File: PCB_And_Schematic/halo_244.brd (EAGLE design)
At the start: 38.1 x 42.9 mm, 14 parts

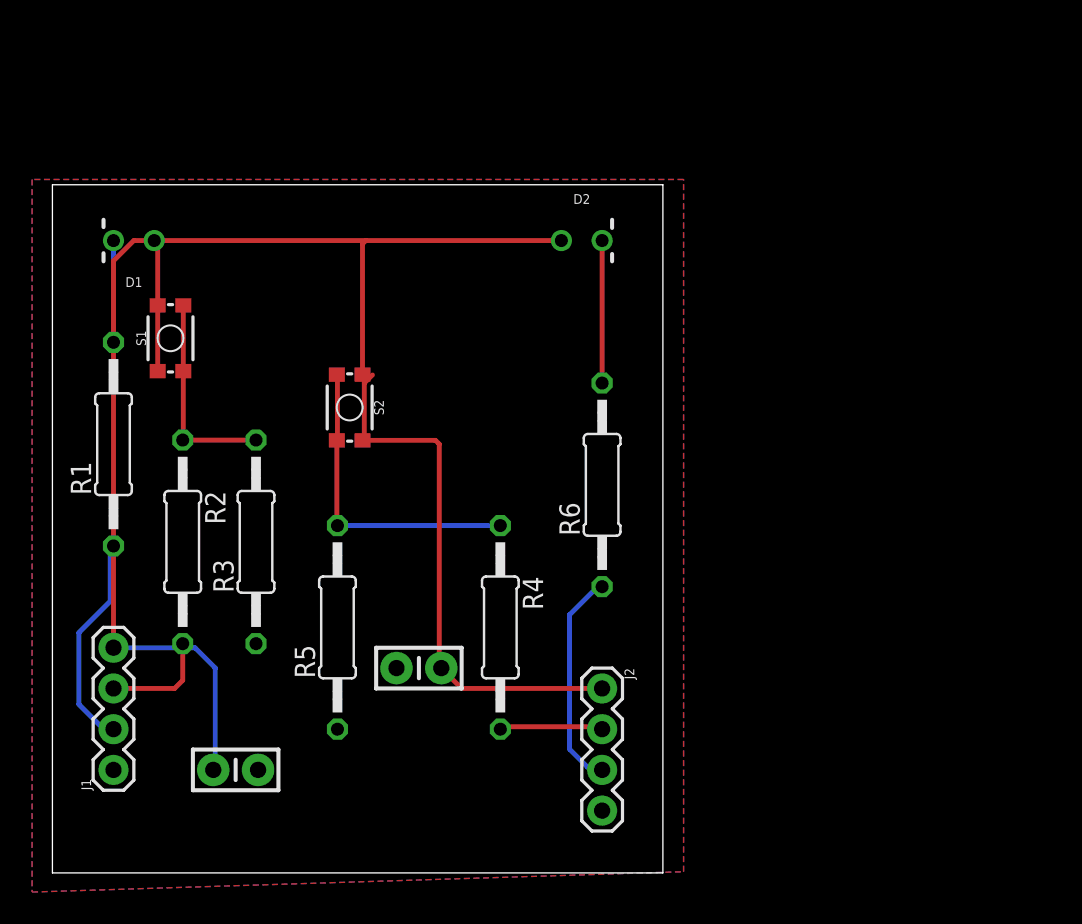
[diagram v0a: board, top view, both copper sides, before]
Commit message: final pcb files
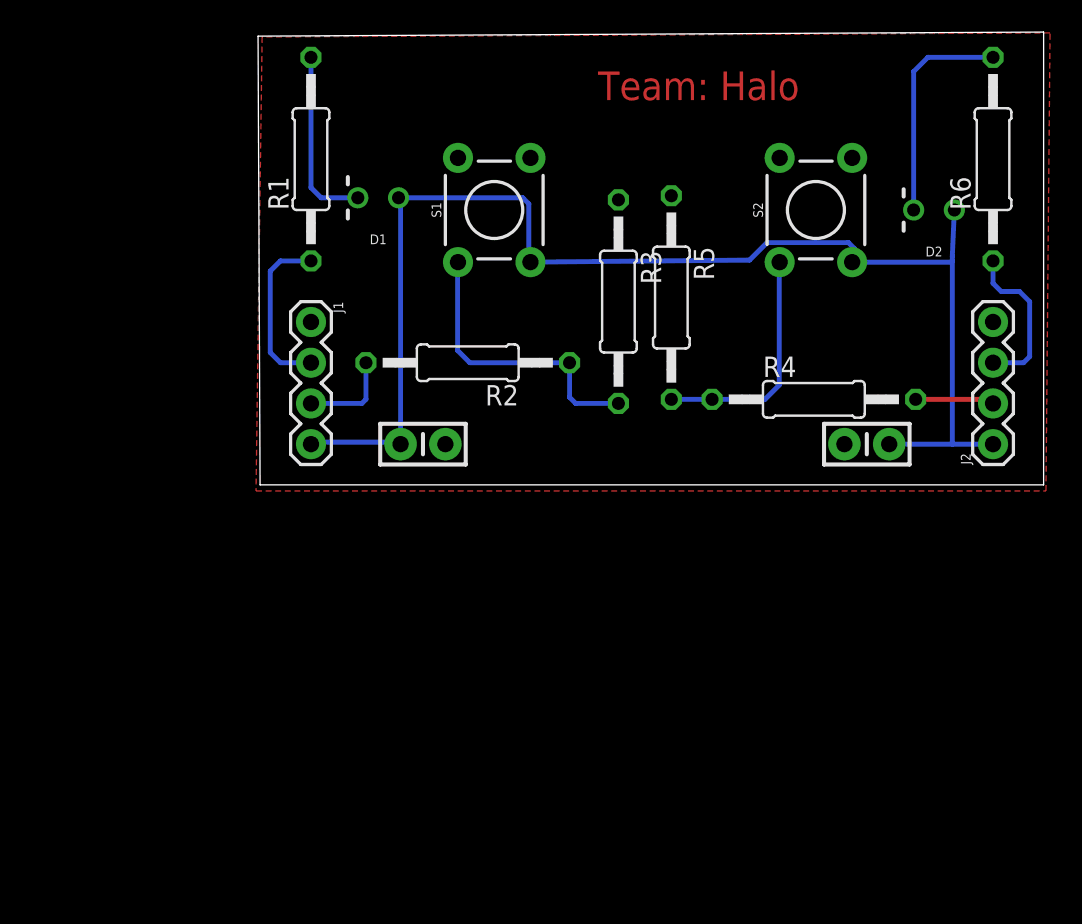
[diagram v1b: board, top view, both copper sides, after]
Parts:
- S1, S2: value (none) -> MOMENTARY-SWITCH-SPST-PTH-6.0MM; device SparkFun-Switches:TACTILE_SWITCH_SMD_4.6X2.8MM -> SparkFun-Switches:TACTILE_SWITCH_PTH_6.0MM
- moved R6 31.7 mm to (58.7, 44.5)
- moved S2 31.6 mm to (47.6, 41.3), turned to 90 degrees
- moved C1 31.2 mm to (50.8, 26.7)
- moved J1 30.5 mm to (16.1, 34.3), turned to 270 degrees
- moved R5 29.3 mm to (38.6, 35.8), turned to 270 degrees
- moved J2 28.8 mm to (58.7, 26.7), turned to 90 degrees
- moved R3 27.1 mm to (35.3, 35.6), turned to 270 degrees
- moved R4 24.2 mm to (47.5, 29.5), turned to 0 degrees
- moved C2 23.4 mm to (23.1, 26.7)
- moved D2 22.1 mm to (55.0, 41.3), turned to 180 degrees
- moved S1 21.7 mm to (27.6, 41.3)
- moved R1 21.6 mm to (16.1, 44.5)
- moved R2 21.0 mm to (25.9, 31.8), turned to 180 degrees
- moved D1 15.5 mm to (20.3, 42.0)
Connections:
- net N$1: no longer S1.2
- net N$4: no longer S2.2
- net VCC: no longer S1.4, S2.4
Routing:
- net VCC: track 120.5 -> 82.9 mm
- net N$1: track 13.0 -> 18.2 mm
- net N$3: track 9.11 -> 14.0 mm
- net N$4: track 19.6 -> 14.8 mm
- net N$2: track 6.56 -> 11.3 mm
- net LED2: track 13.8 -> 10.2 mm
- net LED1: track 13.6 -> 11.0 mm
- net SW2: track 6.50 -> 4.93 mm
- net SW1: track 6.81 -> 5.82 mm
- removed copper zone on layer 16, net GND
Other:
- board size 38.1 x 42.9 mm -> 49 x 28.2 mm
- board text added: "Team: Halo"
